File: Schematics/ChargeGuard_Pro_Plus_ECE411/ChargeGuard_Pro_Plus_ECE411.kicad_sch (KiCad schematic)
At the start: 25 parts, among them J1 Barrel_Jack_MountingPin, J10 Solenoid, J11 Sensor Power, J12 Sensor I2C, J13 OLED Power, J14 OLED I2C, J2 Buck Converter (12V), J3 Buck Converter (5V output), J4 Power Switch, J5 Fan, J6 Reset Switch, J7 Power Push Button, J8 Relay Module Logic, J9 Relay Module Power, Q1 2N3906, Q3 2N7000

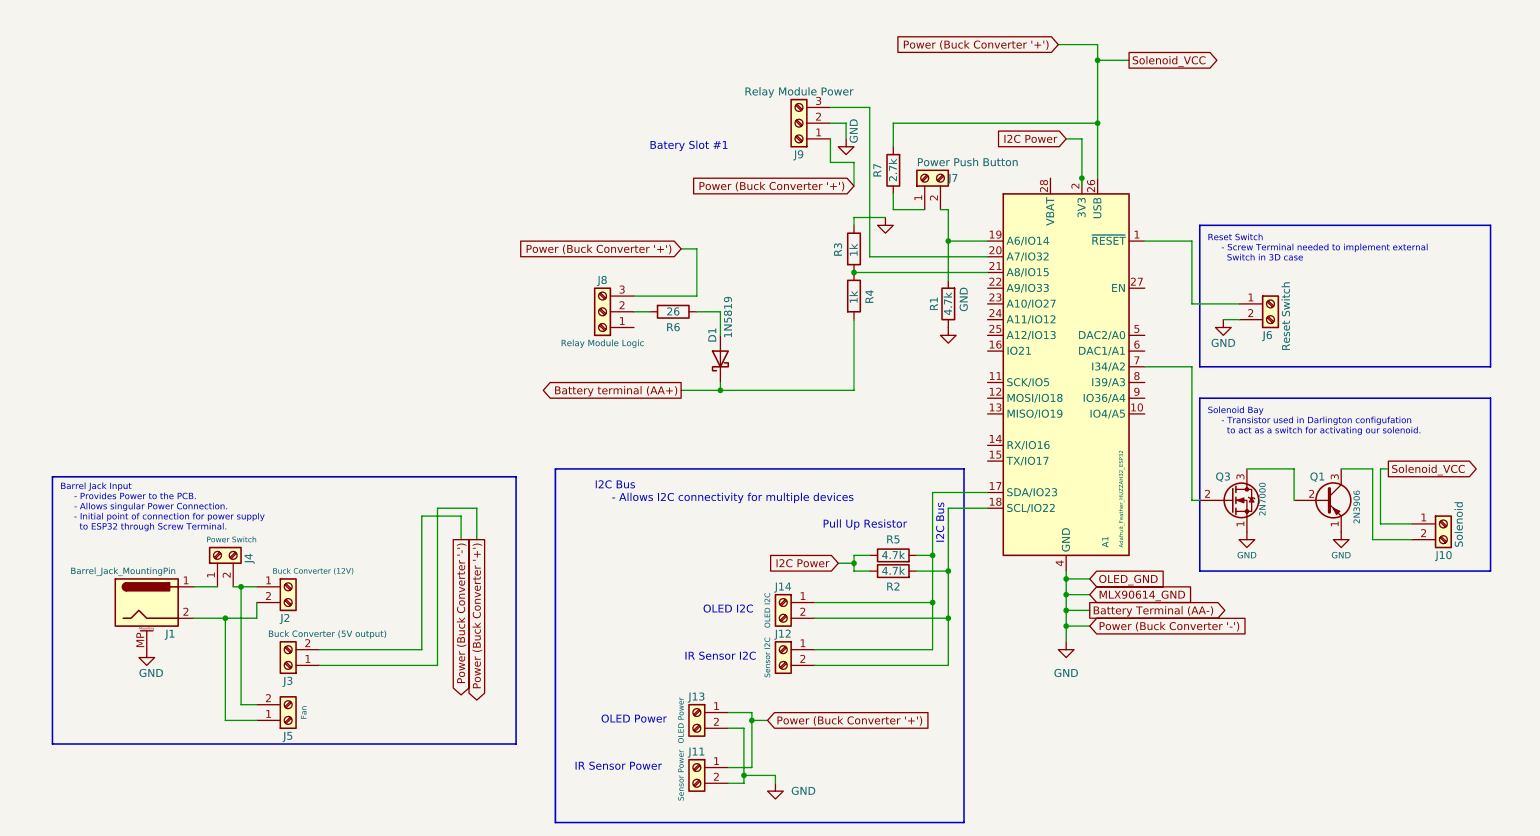
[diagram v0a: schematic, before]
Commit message: ChargeGuard Pro +  - 11/21/2024
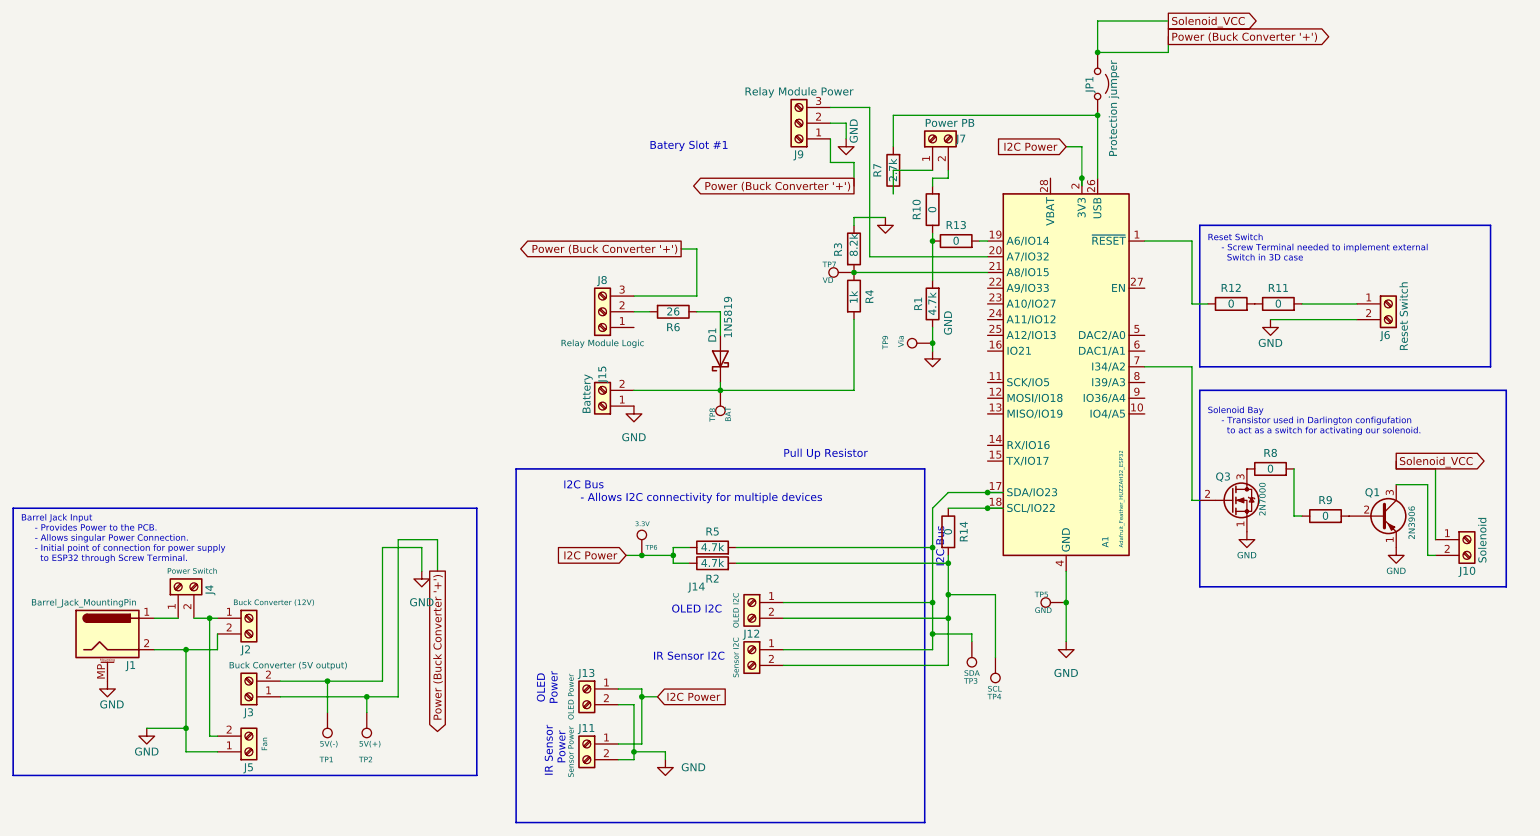
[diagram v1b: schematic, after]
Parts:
- added J15: Battery, TerminalBlock_MetzConnect:TerminalBlock_MetzConnect_Type101_RT01602HBWC_1x02_P5.08mm_Horizontal, symbol Connector:Screw_Terminal_01x02
- added JP1: Protection jumper, TestPoint:TestPoint_2Pads_Pitch2.54mm_Drill0.8mm, symbol Jumper:Jumper_2_Open
- added R10, R11, R12, R13, R14, R8, R9: 0, Resistor_THT:R_Axial_DIN0204_L3.6mm_D1.6mm_P5.08mm_Horizontal, symbol Device:R
- added TP1: 5V(-), Connector_Pin:Pin_D1.0mm_L10.0mm, symbol Connector:TestPoint
- added TP2: 5V(+), Connector_Pin:Pin_D1.0mm_L10.0mm, symbol Connector:TestPoint
- added TP3: SDA, Connector_Pin:Pin_D1.0mm_L10.0mm, symbol Connector:TestPoint
- added TP4: SCL, Connector_Pin:Pin_D1.0mm_L10.0mm, symbol Connector:TestPoint
- added TP5: GND, Connector_Pin:Pin_D1.0mm_L10.0mm, symbol Connector:TestPoint
- added TP6: 3.3V, Connector_Pin:Pin_D1.0mm_L10.0mm, symbol Connector:TestPoint
- added TP7: VD, Connector_Pin:Pin_D1.0mm_L10.0mm, symbol Connector:TestPoint
- added TP8: BAT, Connector_Pin:Pin_D1.0mm_L10.0mm, symbol Connector:TestPoint
- added TP9: Via, Connector_Pin:Pin_D1.0mm_L10.0mm, symbol Connector:TestPoint
- J7: value Power Push Button -> Power PB
- R1, R2, R4, R5, R7: footprint Resistor_THT:R_Axial_DIN0204_L3.6mm_D1.6mm_P5.08mm_Horizontal -> Resistor_SMD:R_1206_3216Metric
- R3: value 1k -> 8.2k; footprint Resistor_THT:R_Axial_DIN0204_L3.6mm_D1.6mm_P5.08mm_Horizontal -> Resistor_SMD:R_1206_3216Metric
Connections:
- net GND: now also J1.2, J2.2 (Pin_2), J5.1 (Pin_1), J15.1 (Pin_1), TP1.1, TP5.1, TP9.1
- net I2C Power: now also J11.1 (Pin_1), J13.1 (Pin_1), TP6.1
- net Power (Buck Converter '+'): now also JP1.1 (A), TP2.1; no longer A1.26 (USB), J11.1 (Pin_1), J13.1 (Pin_1), R7.2
- net at J6.1 (Pin_1): now also R11.2; no longer A1.1 (~{RESET})
- net at J12.1 (Pin_1), J14.1 (Pin_1), R5.2: now also TP3.1; no longer A1.17 (SDA/IO23)
- net at J12.2 (Pin_2), J14.2 (Pin_2), R2.2: now also R14.2, TP4.1; no longer A1.18 (SCL/IO22)
- net at A1.21 (A8/IO15), R3.2, R4.1: now also TP7.1
- net at Q3.3 (D): now also R8.1; no longer Q1.2 (B)
- net Battery terminal (AA+): no longer names the net of D1.1 (K), R4.2
- net Battery terminal (AA+): now also J15.2 (Pin_2), TP8.1
- new net: A1.1 (~{RESET}), R12.1
- new net: R11.1, R12.2
- new net: R1.2, R10.1, R13.1
- new net: A1.18 (SCL/IO22), R14.1
- new net: A1.19 (A6/IO14), R13.2
- new net: A1.26 (USB), JP1.2 (B), R7.2
- new net: J7.2 (Pin_2), R10.2
- new net: R8.2, R9.1
- new net: Q1.2 (B), R9.2
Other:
- moved on the sheet: J1, J10, J11, J12, J13, J14, J2, J3, J4, J5, J6, J7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
